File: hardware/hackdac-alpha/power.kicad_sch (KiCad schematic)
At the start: 50 parts, among them J10 HOLE, J11 HOLE, J12 EXT POWER, J5 EXT 5V, J6 HOLE, J7 HOLE, J8 HOLE, J9 HOLE, P3 P20, P4 P28, Q6 IRLML2244, U10 KF50BDT, U13 LM66200, U14 TPS61170DRVR, U15 TPS63700DRCT, U3 TLE2082

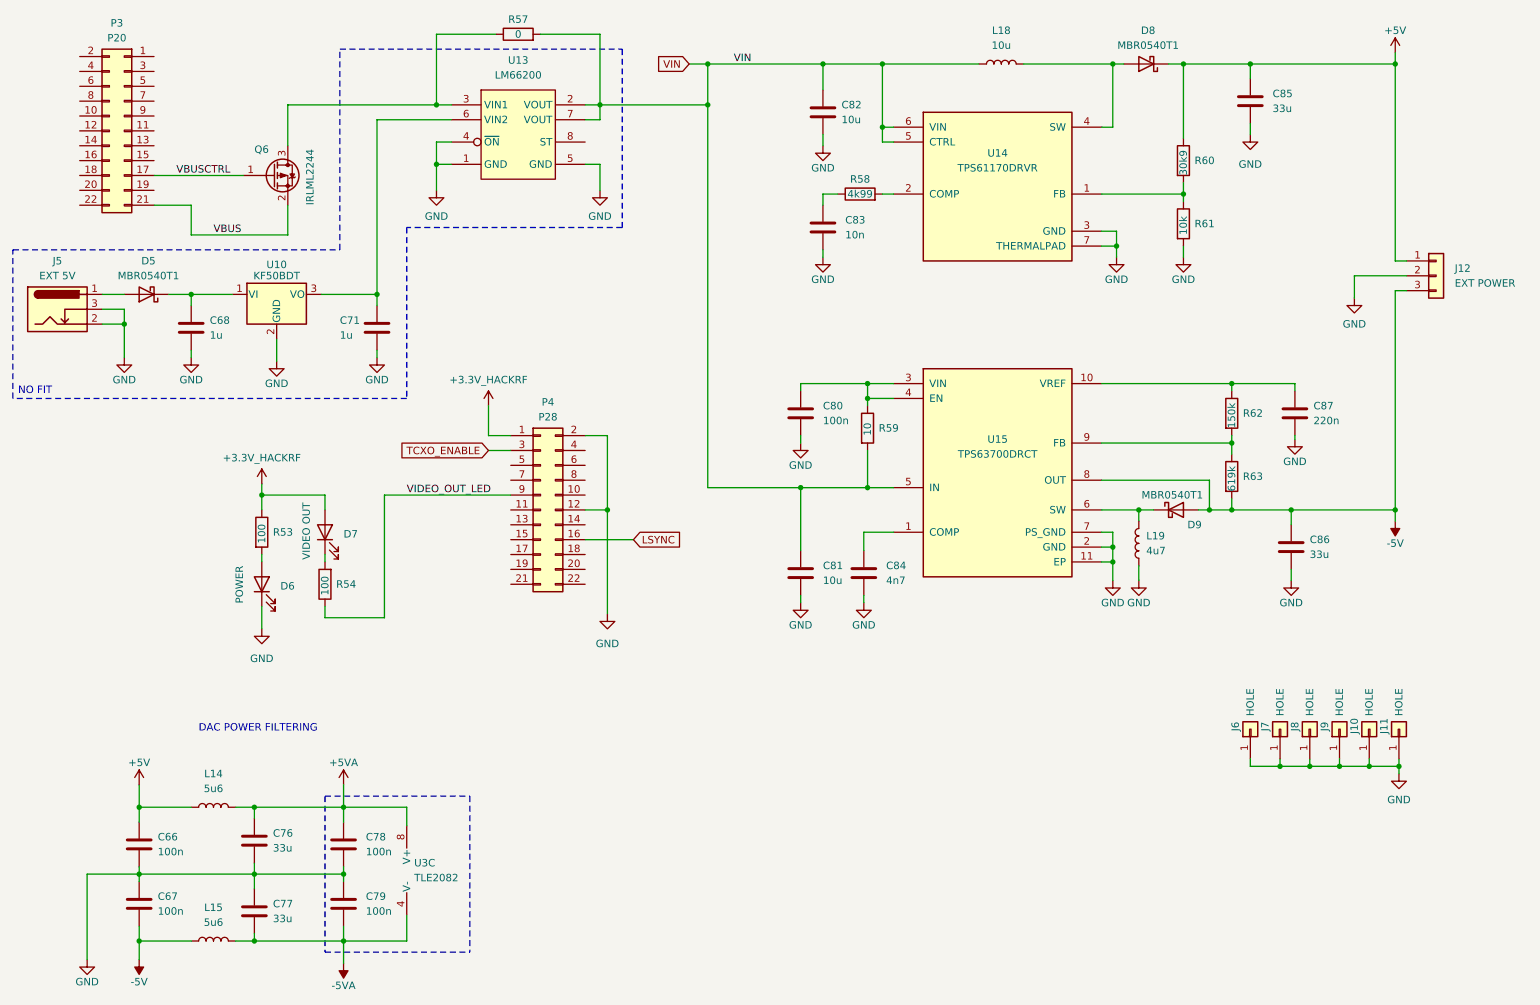
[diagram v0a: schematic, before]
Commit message: Last of major V3 changes
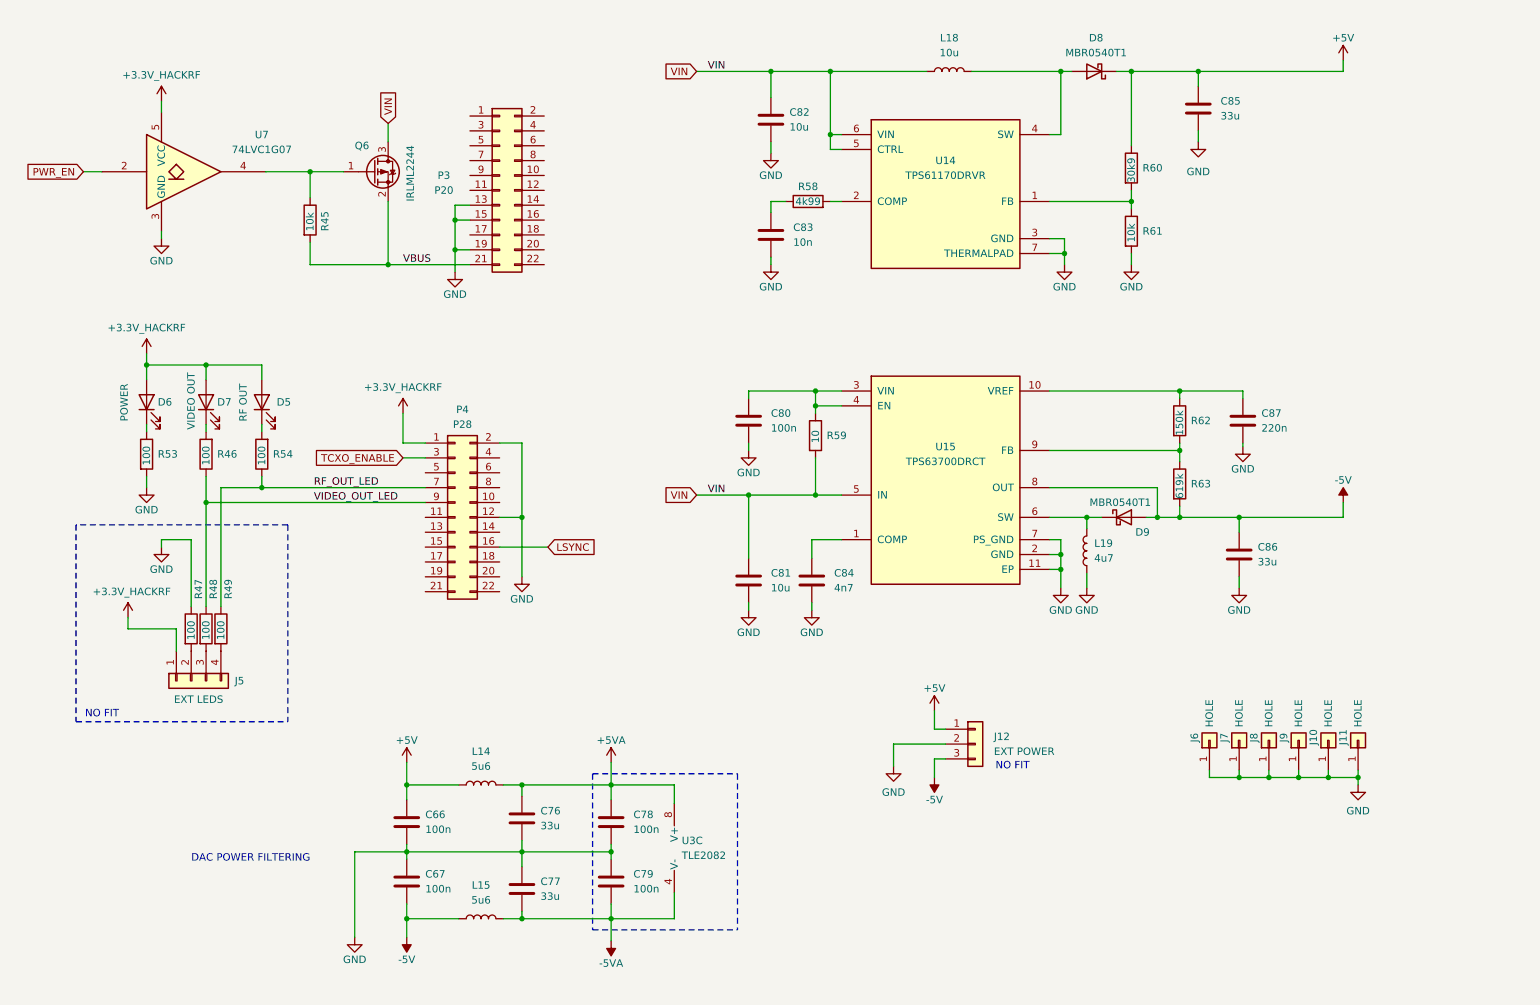
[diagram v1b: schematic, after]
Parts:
- removed C68, C71: 1u, Capacitor_SMD:C_0603_1608Metric, symbol Device:C
- removed D5: MBR0540T1, Diode_SMD:D_SOD-123, symbol Device:D_Schottky
- removed J5: EXT 5V, Connector_BarrelJack:BarrelJack_Horizontal, symbol Connector:Barrel_Jack_Switch
- removed R57: 0, Resistor_SMD:R_0603_1608Metric, symbol Device:R
- removed U10: KF50BDT, Package_TO_SOT_SMD:TO-252-2, symbol Regulator_Linear:KF33BDT
- removed U13: LM66200, Package_TO_SOT_SMD:SOT-583-8, symbol LM66200:LM66200
- added D5: RF OUT, LED_SMD:LED_0805_2012Metric, symbol Device:LED
- added J5: EXT LEDS, symbol Connector_Generic:Conn_01x04
- added R45: 10k, symbol Device:R
- added R46: 100, Resistor_SMD:R_0603_1608Metric, symbol Device:R
- added R47, R48, R49: 100, symbol Device:R
- added U7: 74LVC1G07, symbol 74xGxx:74LVC1G07
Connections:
- net +3.3V_HACKRF: now also D6.2 (A), D5.2 (A), J5.1 (Pin_1), U7.5 (VCC); no longer R53.1
- net GND: now also P3.13 (Pin_13), P3.15 (Pin_15), P3.19 (Pin_19), R53.2, R47.1, U7.3 (GND); no longer D6.1 (K)
- net VBUS: now also R45.2
- net VIDEO_OUT_LED: now also R46.1, R48.1; no longer R54.1
- net VIN: now also Q6.3 (D)
- net at D7.1 (K): now also R46.2; no longer R54.2
- net RF_OUT_LED: now reaches P4.7 (Pin_7)
- net RF_OUT_LED: now also R54.1, R49.1
- net VBUSCTRL: no longer names the net of Q6.1 (G)
- net VBUSCTRL: now also R45.1, U7.4; no longer P3.17 (Pin_17)
- new net: J5.2 (Pin_2), R47.2
- new net: D6.1 (K), R53.1
- new net: J5.3 (Pin_3), R48.2
- new net: J5.4 (Pin_4), R49.2
- new net: D5.1 (K), R54.2
- new net PWR_EN: U7.2
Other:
- moved on the sheet: C66, C67, C76, C77, C78, C79, C80, C81, C82, C83, C84, C85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
